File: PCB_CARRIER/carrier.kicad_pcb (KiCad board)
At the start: 6 copper layers, 69.6 x 46 mm, 97 parts, among them J1 SODIMM-260_Split, J2 Micro_SD_Card_Det2, Q2 BSS138, Q3 BSS138, Q4 BC817-40, Q5 BSS138, SW1 SW_DIP_x04, U1 SN74LVC8T245, U2 SN74LVC8T245, U3 SN74LVC8T245, U4 RT9742GGJ5

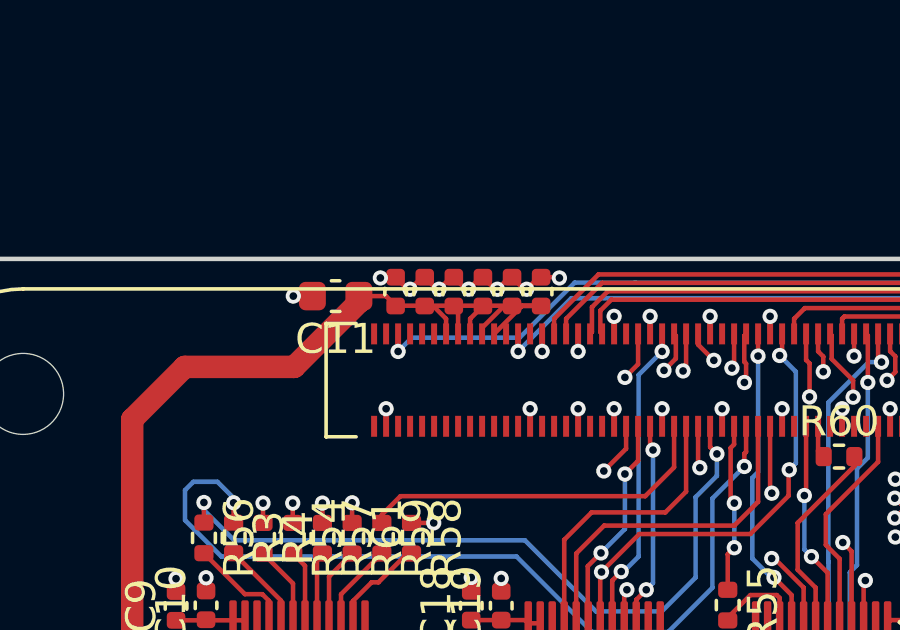
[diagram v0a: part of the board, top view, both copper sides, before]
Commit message: adding power to the journal
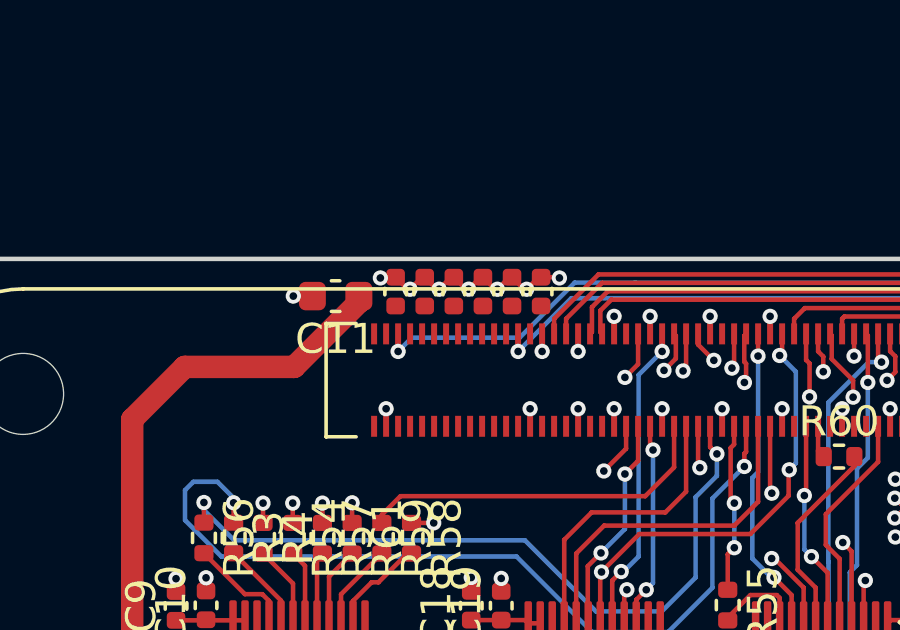
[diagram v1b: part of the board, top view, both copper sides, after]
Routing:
- net +5V: track 106.8 -> 93.7 mm
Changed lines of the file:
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@@
-	)
-	(segment
-		(start 124.812501 56.500025)
-		(end 124.812501 55.997625)
-		(width 0.1524)
-		(layer "F.Cu")
-		(net 33)
 	)
 	(segment
@@
 	)
 	(segment
-		(start 121.905 55.24)
-		(end 122.81 55.24)
-		(width 0.1524)
-		(layer "F.Cu")
-		(net 33)
-	)
-	(segment
 		(start 114.35 59.35)
 		(end 116.1 57.6)
 		(width 0.75)
-		(layer "F.Cu")
-		(net 33)
-	)
-	(segment
-		(start 126.012501 56.297499)
-		(end 126.74 55.57)
-		(width 0.1524)
 		(layer "F.Cu")
 		(net 33)
@@
 		(end 168.1 96.65)
 		(width 0.75)
-		(layer "F.Cu")
-		(net 33)
-	)
-	(segment
-		(start 126.74 55.57)
-		(end 127.01 55.57)
-		(width 0.1524)
-		(layer "F.Cu")
-		(net 33)
-	)
-	(segment
-		(start 124.384876 55.57)
-		(end 124.1 55.57)
-		(width 0.1524)
 		(layer "F.Cu")
 		(net 33)
@@
 	)
 	(segment
-		(start 125.612501 56.500025)
-		(end 125.612501 55.997499)
-		(width 0.1524)
-		(layer "F.Cu")
-		(net 33)
-	)
-	(segment
-		(start 127.97 55.56)
-		(end 127.98 55.57)
-		(width 0.1524)
-		(layer "F.Cu")
-		(net 33)
-	)
-	(segment
-		(start 125.612501 55.997499)
-		(end 126.04 55.57)
-		(width 0.1524)
-		(layer "F.Cu")
-		(net 33)
-	)
-	(segment
 		(start 144.4 79.25)
 		(end 144.4 70.55)
 		(width 0.75)
-		(layer "F.Cu")
-		(net 33)
-	)
-	(segment
-		(start 123.13 55.56)
-		(end 127.97 55.56)
-		(width 0.1524)
 		(layer "F.Cu")
 		(net 33)
@@
 	)
 	(segment
-		(start 125.212501 56.500025)
-		(end 125.212501 55.712501)
-		(width 0.1524)
-		(layer "F.Cu")
-		(net 33)
-	)
-	(segment
 		(start 142.75 68.9)
 		(end 115.5 68.9)
 		(width 0.75)
-		(layer "F.Cu")
-		(net 33)
-	)
-	(segment
-		(start 126.412501 56.500025)
-		(end 127.342526 55.57)
-		(width 0.1524)
-		(layer "F.Cu")
-		(net 33)
-	)
-	(segment
-		(start 124.812501 55.997625)
-		(end 124.384876 55.57)
-		(width 0.1524)
-		(layer "F.Cu")
-		(net 33)
-	)
-	(segment
-		(start 125.212501 55.712501)
-		(end 125.07 55.57)
-		(width 0.1524)
-		(layer "F.Cu")
-		(net 33)
-	)
-	(segment
-		(start 122.81 55.24)
-		(end 123.13 55.56)
-		(width 0.1524)
 		(layer "F.Cu")
 		(net 33)
@@
 		(layer "F.Cu")
 		(net 33)
-	)
-	(segment
-		(start 126.012501 56.500025)
-		(end 126.012501 56.297499)
-		(width 0.1524)
-		(layer "F.Cu")
-		(net 33)
-	)
-	(segment
-		(start 127.342526 55.57)
-		(end 127.98 55.57)
-		(width 0.1524)
-		(layer "F.Cu")
-		(net 33)
